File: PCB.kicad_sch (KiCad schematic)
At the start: 69 parts, among them J1 USB_C_Receptacle_USB2.0_16P, J10 Conn_01x03_Pin, J2 Conn_01x03_Pin, J3 USB_C_Receptacle_USB2.0_16P, J4 Conn_01x08_Socket, J5 Conn_01x02_Pin, J6 Conn_01x04_Pin, J7 Conn_01x07_Pin, J9 Conn_01x03_Pin, Q1 S8050, Q2 S8050, SW1 SW_Push, SW2 SW_Push, SW3 SW_Push, SW4 SW_Push, SW5 SW_Push, SW6 RotaryEncoder_Switch_MP, U1 CH340C, U2 USBLC6-2SC6, U3 USBLC6-2SC6, U4 AMS1117-3.3 (UMW), U6 ESP32-S3-WROOM-1

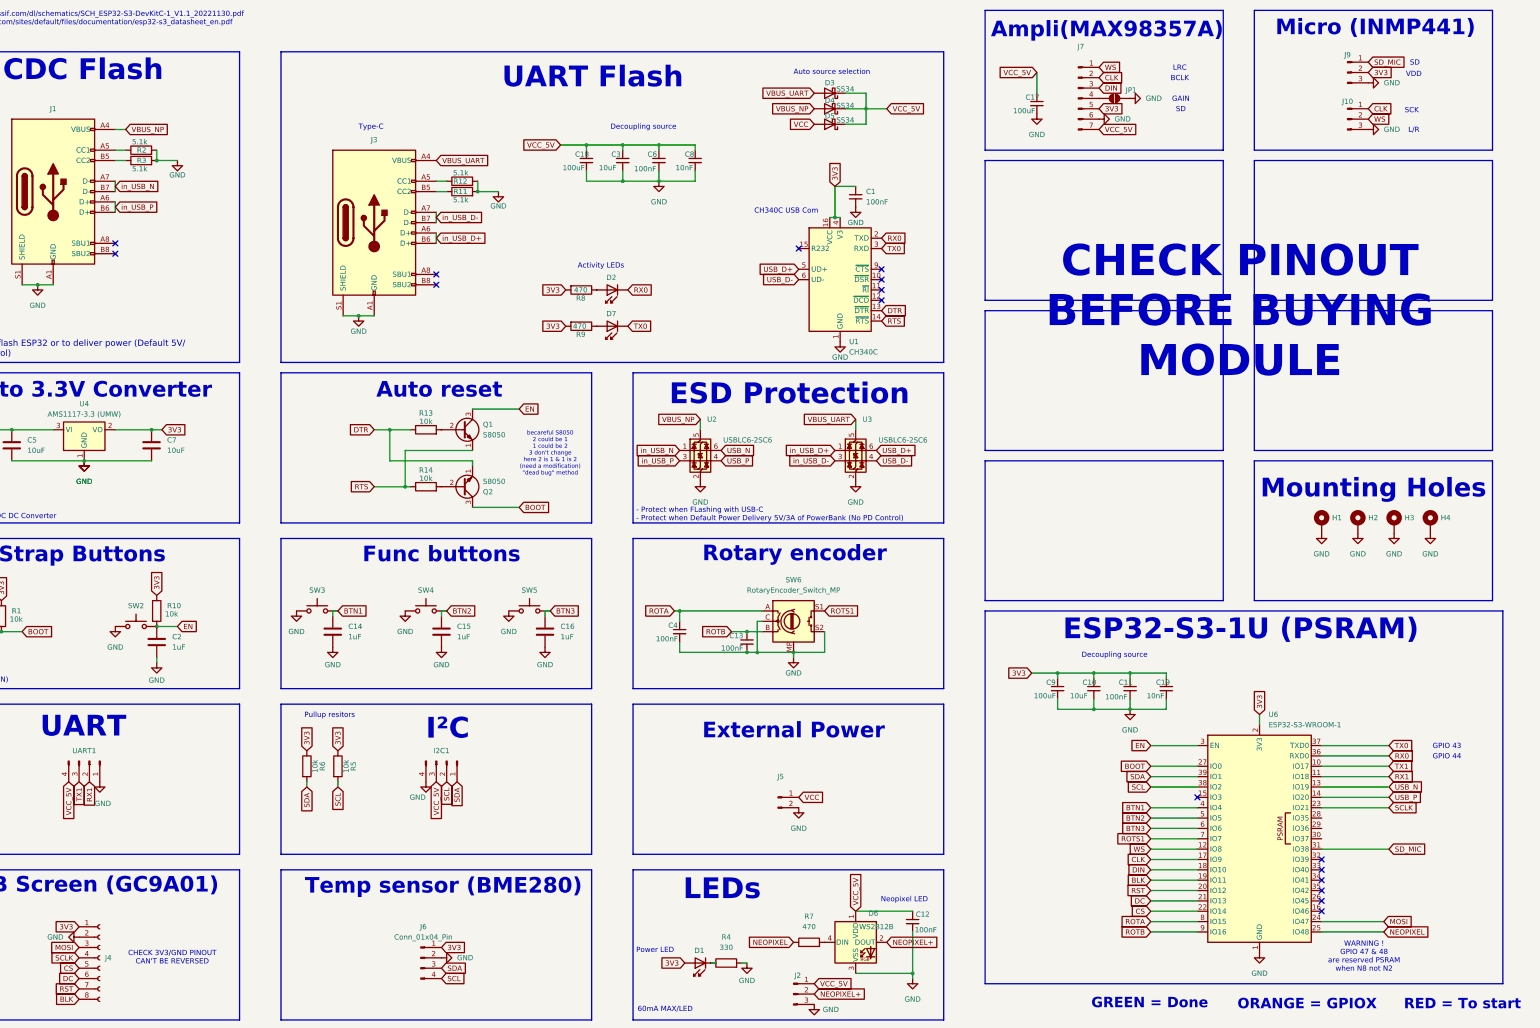
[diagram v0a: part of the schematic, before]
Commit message: update V2
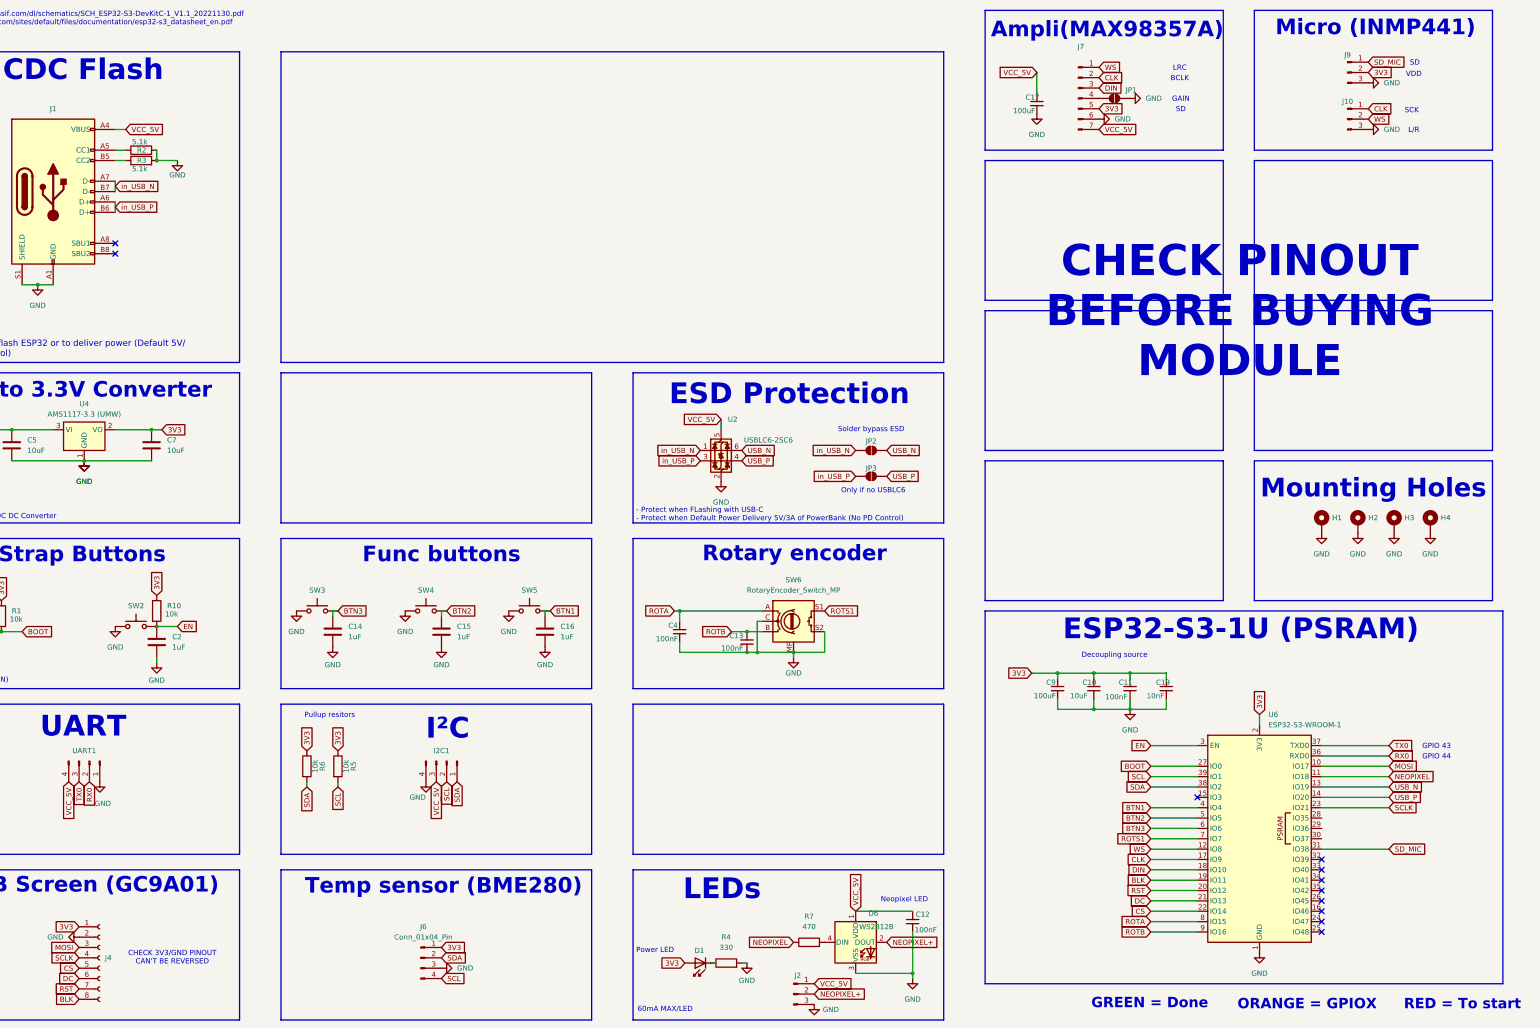
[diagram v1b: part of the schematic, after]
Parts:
- removed C1, C6: 100nF, Capacitor_SMD:C_0805_2012Metric_Pad1.18x1.45mm_HandSolder, symbol Device:C_Small
- removed C18: 100uF, Capacitor_SMD:C_1210_3225Metric_Pad1.33x2.70mm_HandSolder, symbol Device:C_Small
- removed C3: 10uF, Capacitor_SMD:C_0805_2012Metric_Pad1.18x1.45mm_HandSolder, symbol Device:C_Small
- removed C8: 10nF, Capacitor_SMD:C_0805_2012Metric_Pad1.18x1.45mm_HandSolder, symbol Device:C_Small
- removed D2, D7: ~, LED_SMD:LED_0805_2012Metric_Pad1.15x1.40mm_HandSolder, symbol LED:SFH482
- removed D3, D4, D5: SS34, Diode_SMD:D_SMA_Handsoldering, symbol Device:D_Schottky
- removed J3: USB_C_Receptacle_USB2.0_16P, Connector_USB:USB_C_Receptacle_HRO_TYPE-C-31-M-12, symbol Connector:USB_C_Receptacle_USB2.0_16P
- removed J5: Conn_01x02_Pin, Connector_PinHeader_2.54mm:PinHeader_1x02_P2.54mm_Vertical, symbol Connector:Conn_01x02_Pin
- removed Q1, Q2: S8050, Package_TO_SOT_SMD:SOT-23-3, symbol Transistor_BJT:S8050
- removed R11, R12: 5.1k, Resistor_SMD:R_0805_2012Metric_Pad1.20x1.40mm_HandSolder, symbol Device:R
- removed R13, R14: 10k, Resistor_SMD:R_1206_3216Metric_Pad1.30x1.75mm_HandSolder, symbol Device:R
- removed R8, R9: 470, Resistor_SMD:R_0805_2012Metric_Pad1.20x1.40mm_HandSolder, symbol Device:R
- removed U1: CH340C, Package_SO:SOIC-16_3.9x9.9mm_P1.27mm, symbol Interface_USB:CH340C
- removed U3: USBLC6-2SC6, Package_TO_SOT_SMD:SOT-23-6_Handsoldering, symbol Power_Protection:USBLC6-2SC6
- added JP2, JP3: SolderJumper_2_Open, Jumper:SolderJumper-2_P1.3mm_Open_RoundedPad1.0x1.5mm, symbol Jumper:SolderJumper_2_Open
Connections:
- net VBUS_NP is gone; now on net VCC_5V: J1.A4 (VBUS), J1.A9 (VBUS), J1.B4 (VBUS), J1.B9 (VBUS), U2.5 (VBUS)
- net BTN1: now also C16.1, SW5.2; no longer C14.1, SW3.2
- net BTN3: now also C14.1, SW3.2; no longer C16.1, SW5.2
- net GND: now also J6.3 (Pin_3); no longer J6.2 (Pin_2)
- net MOSI: now also U6.10 (IO17); no longer U6.24 (IO47)
- net NEOPIXEL: now also U6.11 (IO18); no longer U6.25 (IO48)
- net RX0: now also UART1.2 (Pin_2)
- net SCL: now also U6.39 (IO1); no longer U6.38 (IO2)
- net SDA: now also J6.2 (Pin_2), U6.38 (IO2); no longer J6.3 (Pin_3), U6.39 (IO1)
- net TX0: now also UART1.3 (Pin_3)
- net USB_N: now also JP2.2 (B)
- net USB_P: now also JP3.2 (B)
- net in_USB_N: now also JP2.1 (A)
- net in_USB_P: now also JP3.1 (A)
- removed net RX1: U6.11 (IO18), UART1.2 (Pin_2)
- removed net TX1: U6.10 (IO17), UART1.3 (Pin_3)
- no-connect marks 16 -> 11
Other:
- note added: "Only if no USBLC6"
- note added: "Solder bypass ESD"
- note removed: "Activity LEDs"
- note removed: "Auto reset"
- note removed: "Auto source selection"
- note removed: "CH340C USB Com"
- note removed: "External Power"
- note removed: "Type-C"
- note removed: "UART Flash"
- note removed: "WARNING ! GPIO 47 & 48 are reserved PSRAM when N8 not N2"
- note removed: "becareful S8050 2 could be 1 1 could be 2 3 don't change here 2 is 1 & 1 is 2 (need a modification) "dead bug" method"
- moved on the sheet: U2
